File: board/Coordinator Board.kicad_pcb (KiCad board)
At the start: 4 copper layers, 45.5 x 39.6 mm, 30 parts, among them J1 Conn_01x04, J2 Conn_01x04, J3 Conn_01x04, P4 SERIAL, SW1 Switch_SPDT_x2, SW2 Switch_DPST, U0 10118194, U1 LM3671, U2 CD74HC4050, U3 ESP-12E, U4 DIY-OLED-0.96, U5 SF303GJ26, U6 SN74LVC1T45, U7 SN74LVC1T45

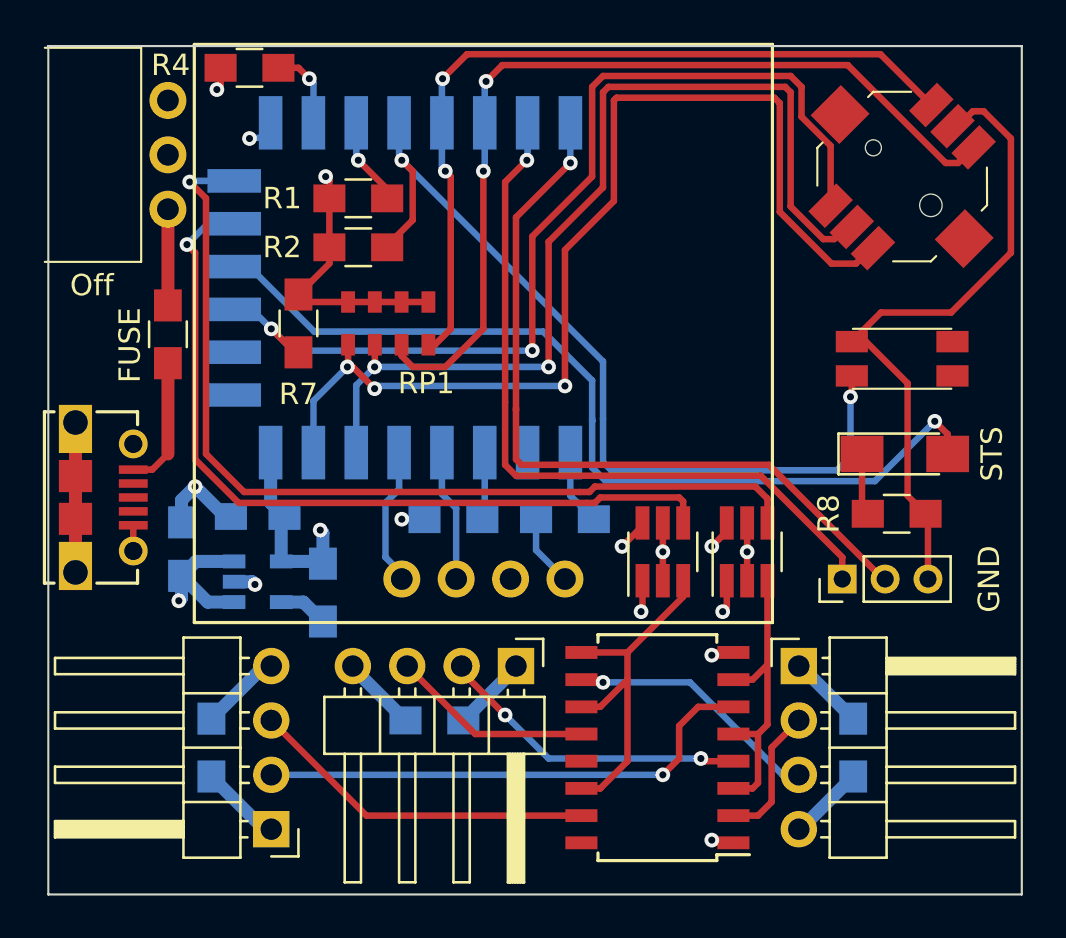
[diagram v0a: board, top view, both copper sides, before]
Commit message: Finished and ordered v3.0 of the board!!
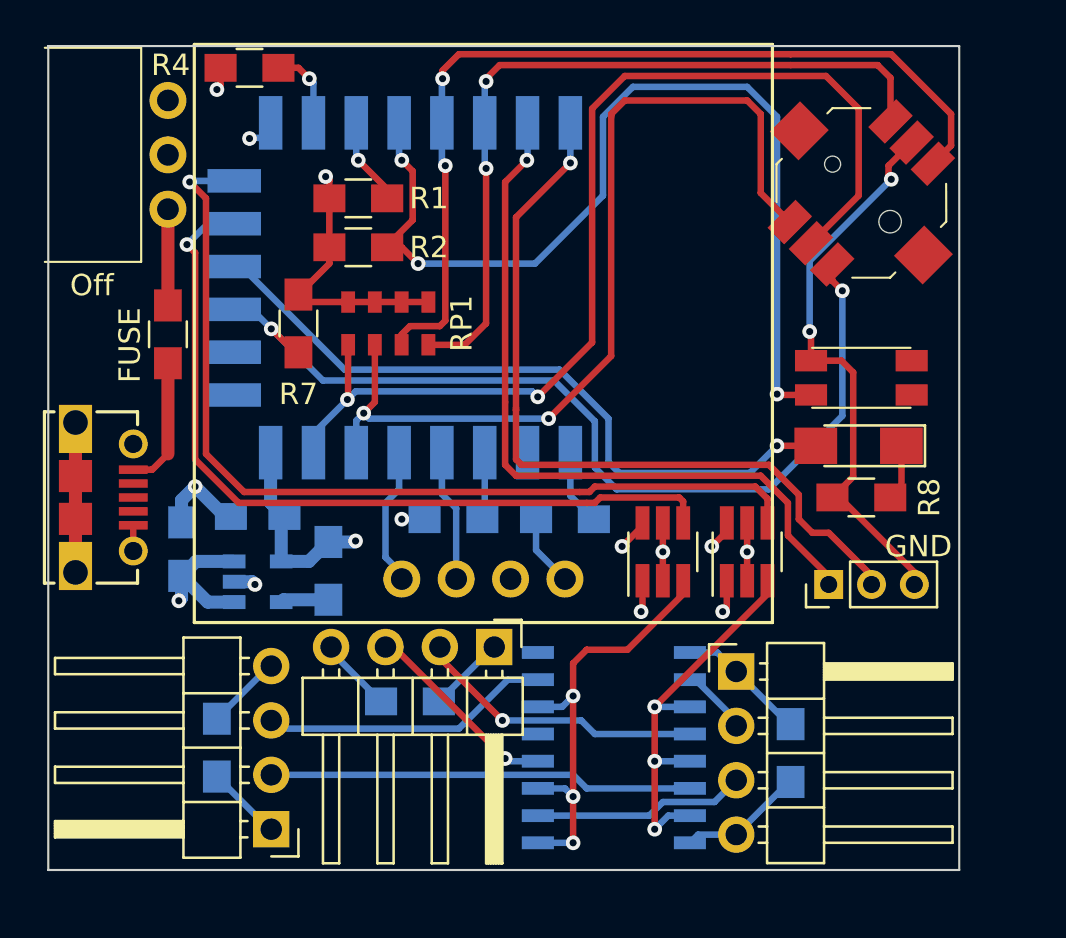
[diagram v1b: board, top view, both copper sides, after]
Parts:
- U2: moved to B.Cu
- moved J3 2.93 mm to (126.1, 132.4)
- moved C6 2.93 mm to (128.6, 136.2)
- moved D1 2.19 mm to (131.8, 121.8), turned to 180 degrees
- moved SW2 2.10 mm to (131.9, 118.7)
- moved U5 2.05 mm to (131.9, 110.0)
- moved U2 2.03 mm to (120.3, 135.9)
- moved R8 1.82 mm to (131.9, 124.2), turned to 180 degrees
- moved C4 1.45 mm to (110.8, 133.8)
- moved J2 1.35 mm to (114.7, 131.2)
- moved L1 1.05 mm to (107.0, 127.7)
- moved P4 0.68 mm to (130.4, 128.3)
- moved C5 0.25 mm to (101.8, 135.9)
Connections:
- U3 pad 13: Net-(RP1-Pad4) -> Net-(RP1-Pad3)
- U3 pad 14: Net-(RP1-Pad3) -> Net-(RP1-Pad4)
- U5 pad 1: Net-(R7-Pad2) -> Net-(RP1-Pad2)
- U5 pad 2: Net-(RP1-Pad2) -> Net-(RP1-Pad1)
- U5 pad 3: Net-(RP1-Pad1) -> Net-(R7-Pad2)
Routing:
- net Net-(D1-Pad2): track 41.6 -> 32.4 mm
- net Net-(R2-Pad1): track 39.6 -> 45.1 mm, vias 2 -> 3
- net Net-(U2-Pad3): track 13.9 -> 19.0 mm, vias 0 -> 3
- net Net-(J1-Pad2): track 23.8 -> 19.8 mm, vias 1 -> 0
- net Net-(U2-Pad11): track 17.0 -> 20.8 mm, vias 0 -> 3
- net GND: track 63.9 -> 60.4 mm, vias 7 -> 8
- net Net-(J3-Pad2): track 6.38 -> 3.21 mm
- net Net-(J1-Pad3): track 16.3 -> 13.6 mm
- net Net-(RP1-Pad2): track 44.7 -> 42.1 mm
- net Net-(R7-Pad2): track 45.5 -> 43.0 mm
- net Net-(J3-Pad3): track 12.0 -> 9.95 mm, vias 1 -> 0
- net Net-(RP1-Pad4): track 37.5 -> 36.0 mm
- net +5V: track 21.9 -> 23.2 mm, vias 4 -> 3
- net Net-(RP1-Pad1): track 48.6 -> 49.6 mm, vias 3 -> 2
- net Net-(J2-Pad2): track 14.7 -> 13.7 mm, vias 2 -> 1
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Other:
- board size 45.5 x 39.6 mm -> 42.5 x 38.5 mm
- board text added: "Raver Lights Hub v3.0 Copyright Bryan Hughes 2018"
- board text removed: "Raver Lights Coordinator v3.0 Copyright Bryan Hughes 2018"
- board text removed: "STS"
